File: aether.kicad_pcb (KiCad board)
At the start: 4 copper layers, 87 x 69.8 mm, 83 parts, among them J1 USB_C_Receptacle_USB2.0, J2 Conn_02x12_Top_Bottom, U1 CP2102N, U2 MCP73871_U, U3 LP2985-3.3, U4 LTC3525-5, U5 LoRa-E5

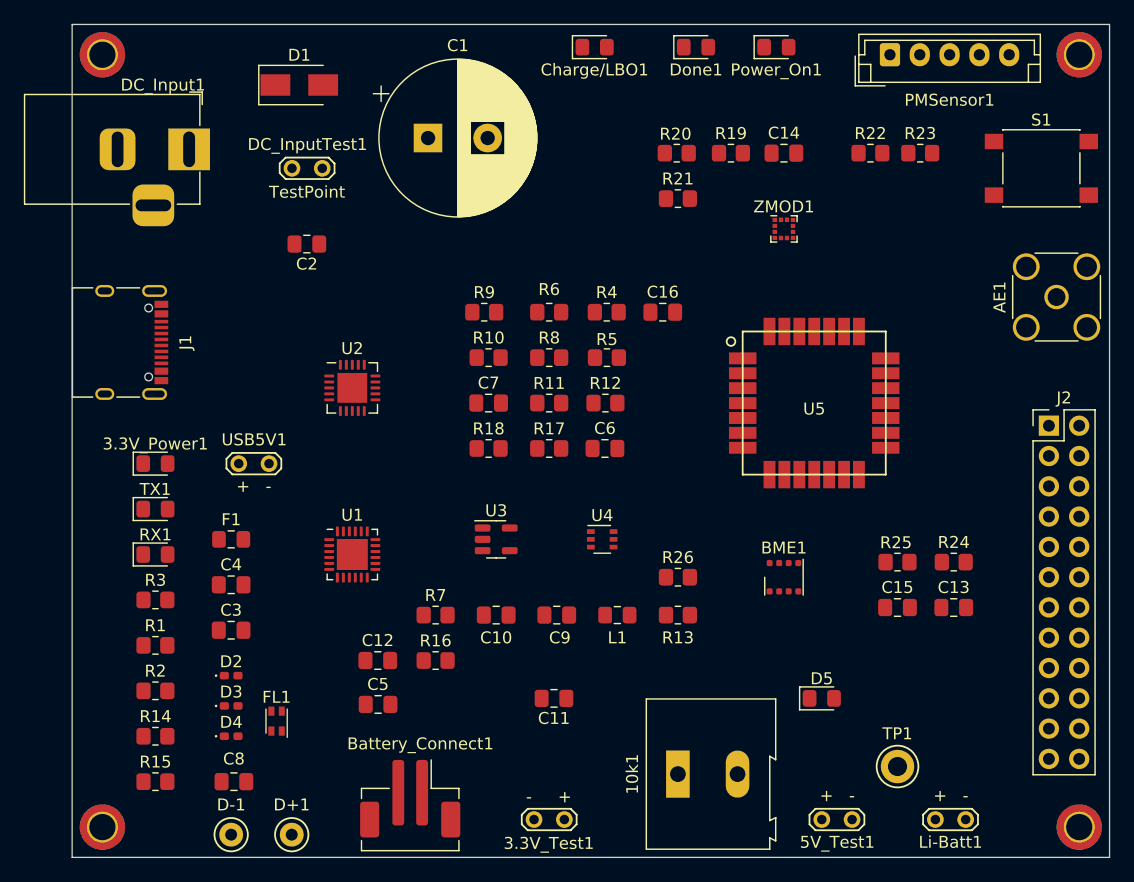
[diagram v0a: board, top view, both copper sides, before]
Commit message: PCB edits
-
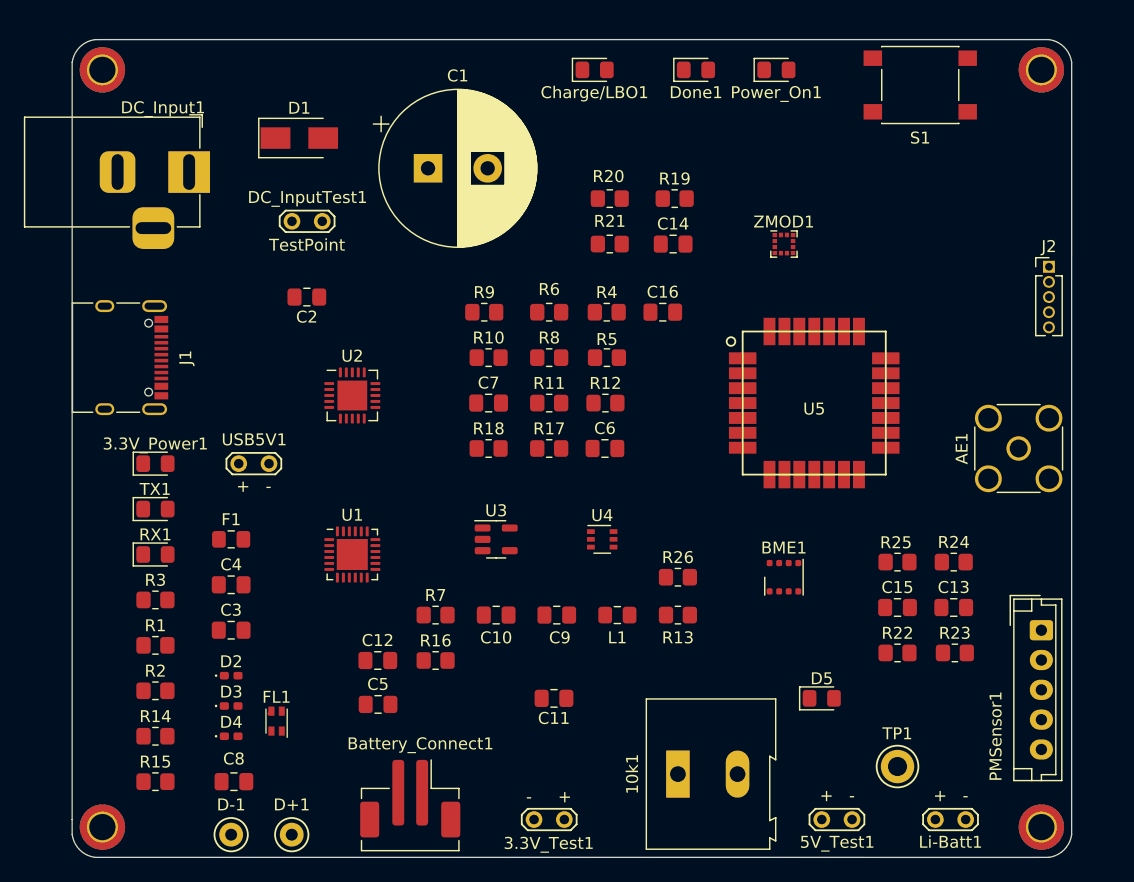
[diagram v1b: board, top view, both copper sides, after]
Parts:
- J2: value Conn_02x12_Top_Bottom -> Conn_01x05; footprint Connector_PinHeader_2.54mm:PinHeader_2x12_P2.54mm_Vertical -> Connector_PinHeader_1.27mm:PinHeader_1x05_P1.27mm_Vertical
- moved PMSensor1 49.9 mm to (184.8, 121.9), turned to -90 degrees
- moved R23 42.0 mm to (177.5, 123.8)
- moved R22 42.0 mm to (172.7, 123.8)
- moved J2 13.3 mm to (185.4, 91.4)
- moved AE1 13.1 mm to (182.9, 106.7)
- moved S1 12.3 mm to (174.6, 76.2)
- moved C14 12.0 mm to (153.9, 89.5)
- moved R21 6.87 mm to (148.6, 89.5)
- moved R20 6.79 mm to (148.6, 85.7)
- moved R19 6.06 mm to (154.0, 85.7)
- moved C2 4.45 mm to (123.2, 94.0)
- moved D1 4.44 mm to (122.6, 80.6)
- moved DC_InputTest1 4.44 mm to (121.9, 87.6)
- moved H3 3.42 mm to (184.8, 74.9)
- moved H1 3.18 mm to (184.8, 138.4)
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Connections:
- J2 pad 1: USB5V -> PA13/SWDIO
- J2 pad 2: +3.3V -> PA14/SWCLK
- J2 pad 3: PA13/SWDIO -> GND
- J2 pad 4: PA14/SWCLK -> RST
- J2 pad 5: RST -> unconnected-(J2-Pad5)
- U5 pad 24: PA13/SCK -> PB13/SCK
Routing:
- net GND: track 0.00 -> 2.19 mm
- net Net-(R15-Pad2): track 0.00 -> 0.97 mm
- added copper zone on In1.Cu, net +3.3V
- added copper zone on In2.Cu, net GND
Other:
- board size 87 x 69.8 mm -> 83.8 x 68.6 mm
